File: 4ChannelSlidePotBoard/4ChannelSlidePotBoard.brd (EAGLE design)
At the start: 98.7 x 64.8 mm, 28 parts

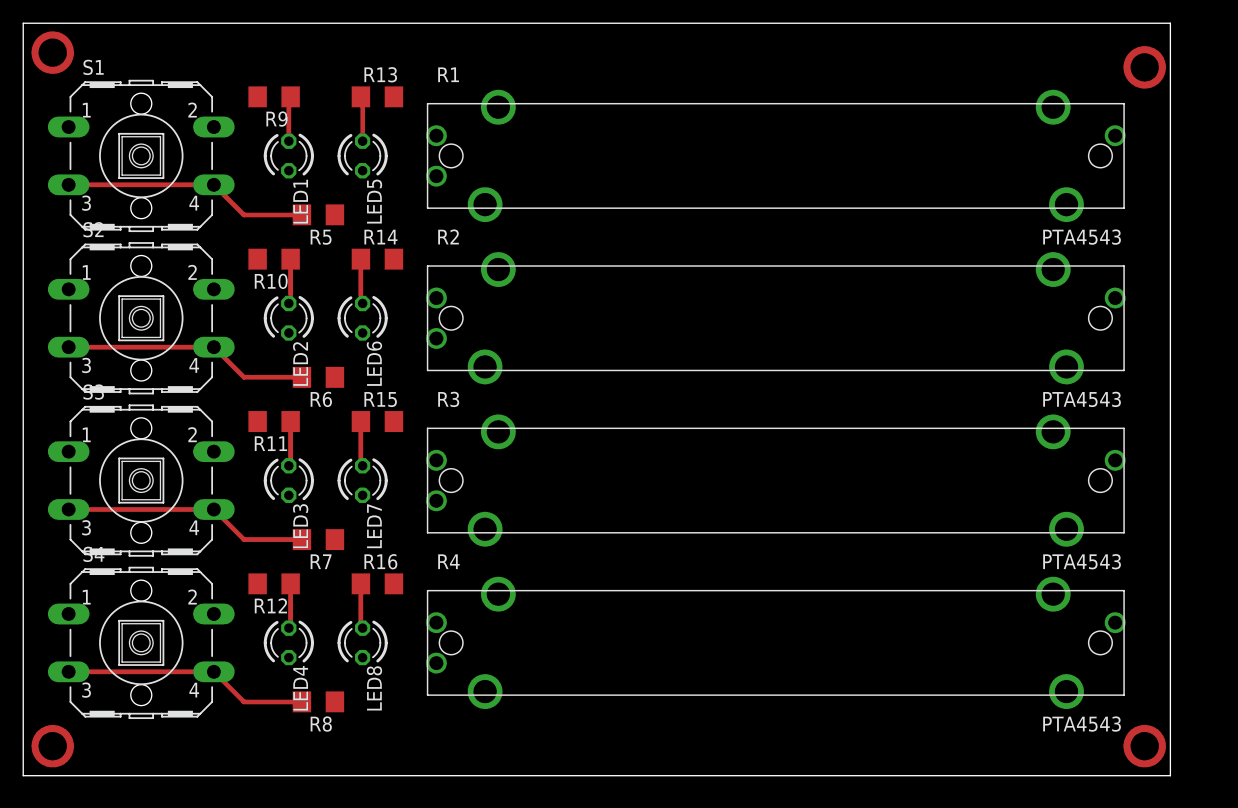
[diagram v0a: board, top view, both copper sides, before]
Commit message: Update to board
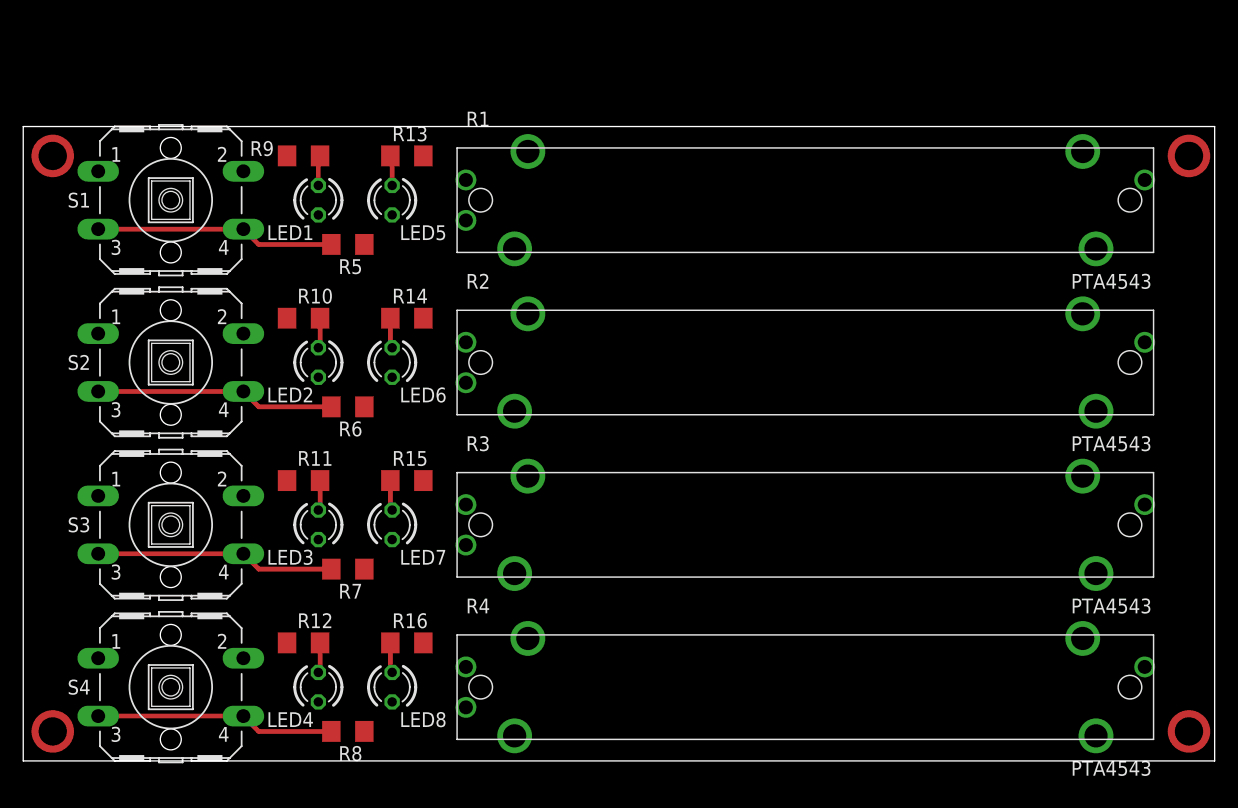
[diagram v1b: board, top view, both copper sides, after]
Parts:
- moved R14 5.68 mm to (33.0, 39.4)
- moved R10 5.68 mm to (24.1, 39.4)
- moved R15 5.68 mm to (33.0, 25.4)
- moved R16 5.68 mm to (33.0, 11.4)
- moved R11 5.68 mm to (24.1, 25.4)
- moved R12 5.68 mm to (24.1, 11.4)
- moved R13 5.68 mm to (33.0, 53.3)
- moved R9 5.68 mm to (24.1, 53.3)
- moved R1 4.58 mm to (67.3, 49.5)
- moved R4 4.58 mm to (67.3, 7.62)
- moved LED1 4.58 mm to (25.4, 49.5)
- moved LED5 4.58 mm to (31.8, 49.5)
- moved S1 4.58 mm to (12.7, 49.5)
- moved R3 4.58 mm to (67.3, 21.6)
- moved R2 4.58 mm to (67.3, 35.6)
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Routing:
- net N$9: track 3.96 -> 2.60 mm
- net N$5: track 3.96 -> 2.60 mm
- net N$6: track 3.87 -> 2.60 mm
- net N$10: track 3.87 -> 2.60 mm
- net N$8: track 3.87 -> 2.60 mm
- net N$12: track 3.87 -> 2.60 mm
- net N$7: track 3.87 -> 2.60 mm
- net N$11: track 3.87 -> 2.60 mm
- net N$2: track 21.2 -> 20.7 mm
- net N$1: track 21.3 -> 20.7 mm
- net N$4: track 21.1 -> 20.6 mm
- net N$3: track 22.5 -> 22.0 mm
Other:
- board size 98.7 x 64.8 mm -> 102.5 x 54.6 mm
